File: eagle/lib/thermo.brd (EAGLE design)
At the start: 160 x 100 mm, 16 parts, among them U2 MLX90640ESF-BAB-000-TU

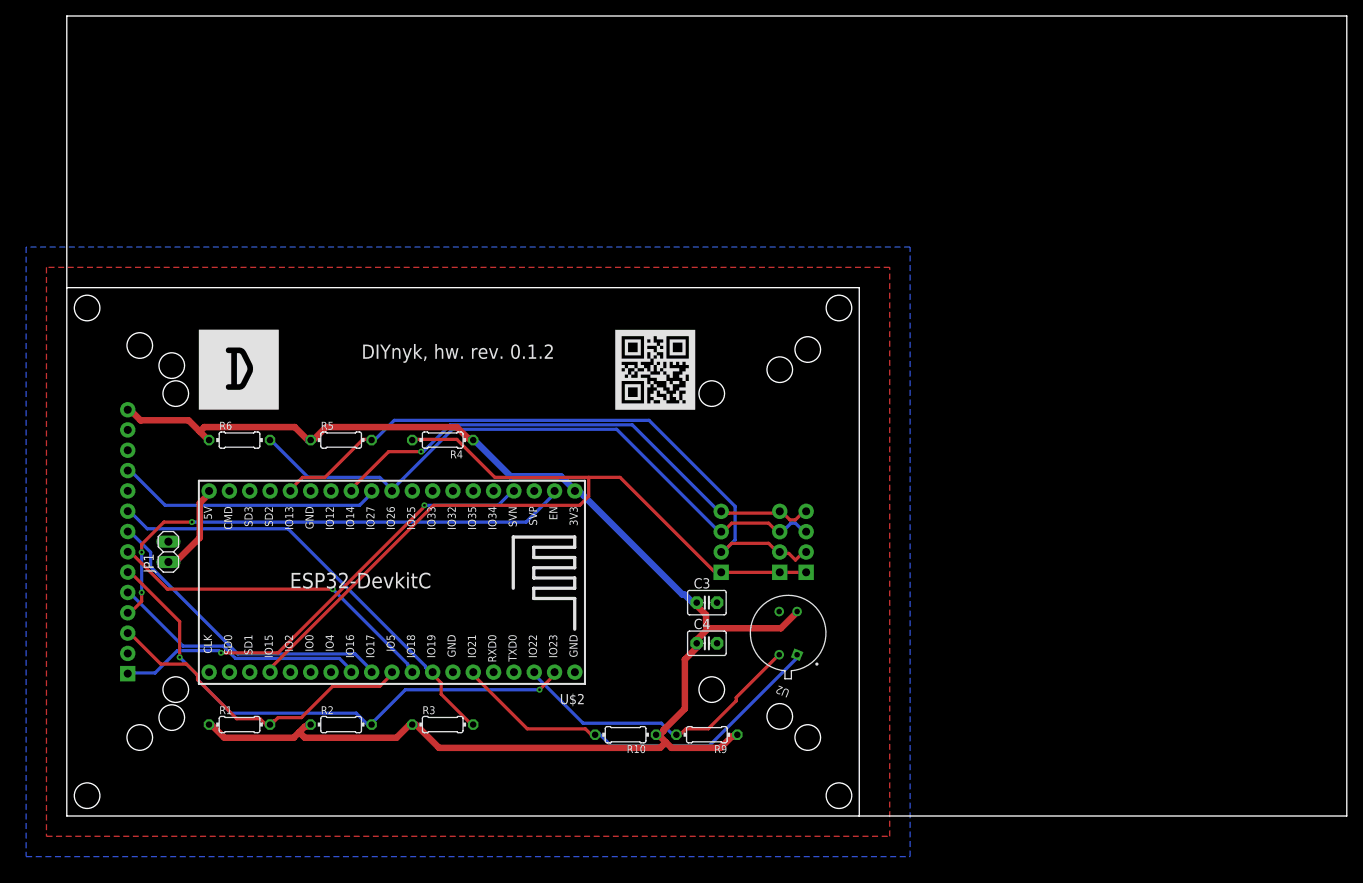
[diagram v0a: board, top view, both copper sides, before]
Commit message: Fixed scheme 0.1.2
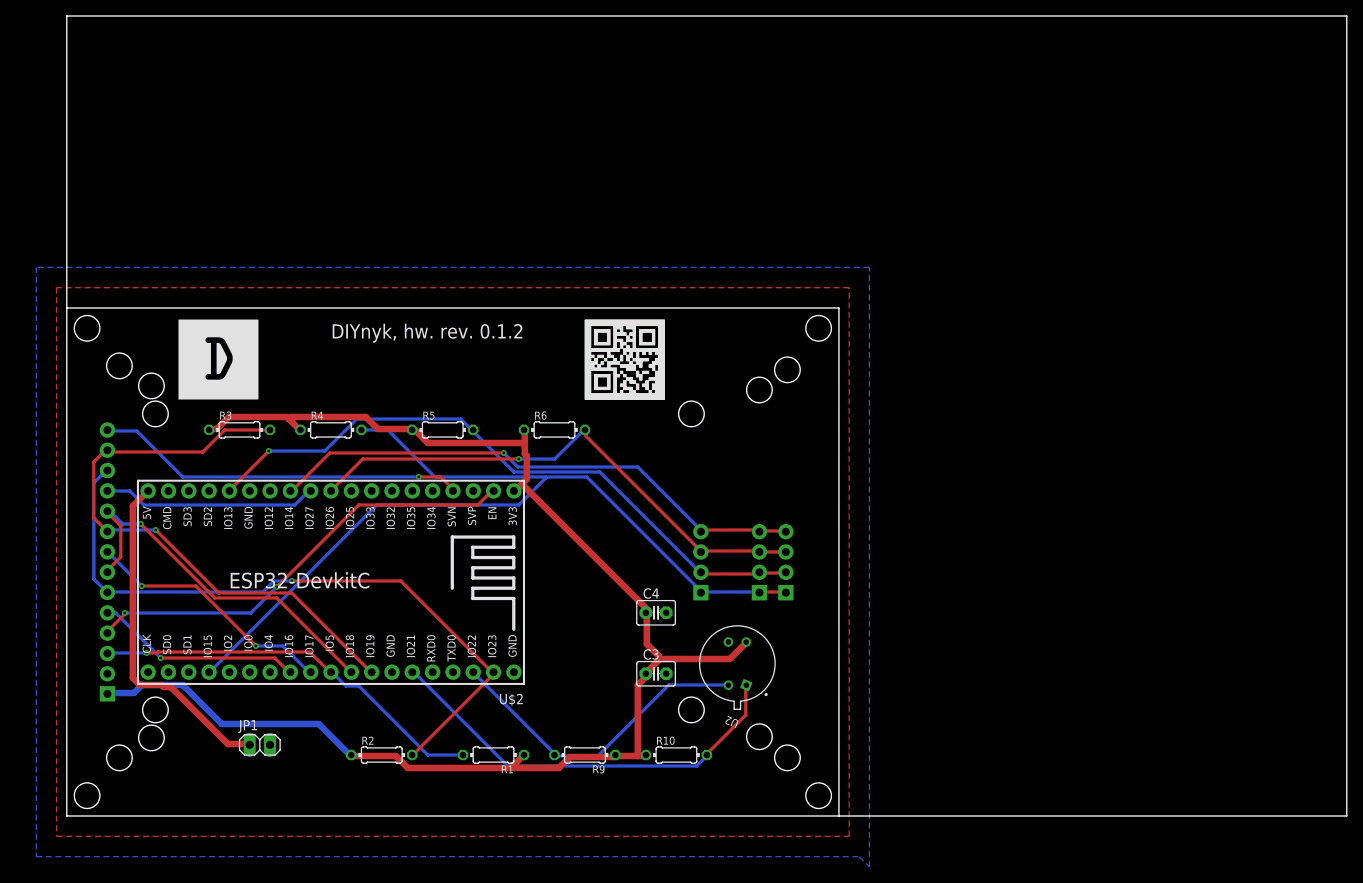
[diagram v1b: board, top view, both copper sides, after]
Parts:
- added U$5: (no value), thermo:QR_10MM
- moved R3 44.7 mm to (21.6, 48.3)
- moved R6 39.4 mm to (61.0, 48.3)
- moved R1 32.0 mm to (53.3, 7.62), turned to 180 degrees
- moved JP1 26.7 mm to (24.1, 8.89), turned to 0 degrees
- moved R9 15.5 mm to (64.8, 7.62)
- moved R4 14.0 mm to (33.0, 48.3), turned to 0 degrees
- moved R5 12.8 mm to (47.0, 48.3)
- moved C3 10.9 mm to (73.7, 17.8)
- moved U$2 7.62 mm to (33.0, 29.2)
- moved C4 7.41 mm to (73.7, 25.4)
- moved U2 7.41 mm to (83.8, 19.1)
- moved R10 6.84 mm to (76.2, 7.62), turned to 0 degrees
- moved R2 6.35 mm to (39.4, 7.62)
- moved U$4 4.02 mm to (64.8, 52.1)
- moved U$1 3.59 mm to (5.08, 48.3)
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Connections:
- net 3V3: now also U$1.VCC!; no longer U$1.TOUCH_IRQ
- net TOUCH_IRQ: now also U$1.TOUCH_IRQ; no longer U$1.VCC!
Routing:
- net +5V: track 11.5 -> 42.3 mm
- net TFT_MISO: track 55.3 -> 73.8 mm, vias 0 -> 1
- net TFT_MOSI: track 67.1 -> 85.0 mm, vias 2 -> 1
- net SD_MISO: track 80.2 -> 67.2 mm, vias 0 -> 1
- net TOUCH_IRQ: track 58.1 -> 46.6 mm, vias 2 -> 1
- net TFT_CS: track 41.0 -> 50.0 mm, vias 0 -> 1
- net 3V3: track 190.6 -> 181.8 mm
- net TFT_RESET: track 64.0 -> 56.0 mm, vias 3 -> 2
- net TFT_LED: track 39.0 -> 31.7 mm, vias 0 -> 2
- net SD_CS: track 107.7 -> 114.1 mm
- net TFT_DC: track 32.2 -> 26.0 mm, vias 0 -> 1
- net TOUCH_CS: track 33.1 -> 27.0 mm
- net TFT_SCK: track 42.0 -> 47.9 mm
- net SDA: track 49.6 -> 53.1 mm
- net SD_SCK: track 66.0 -> 68.6 mm
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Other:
- outline, holes or cut-outs redrawn

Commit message: comleted
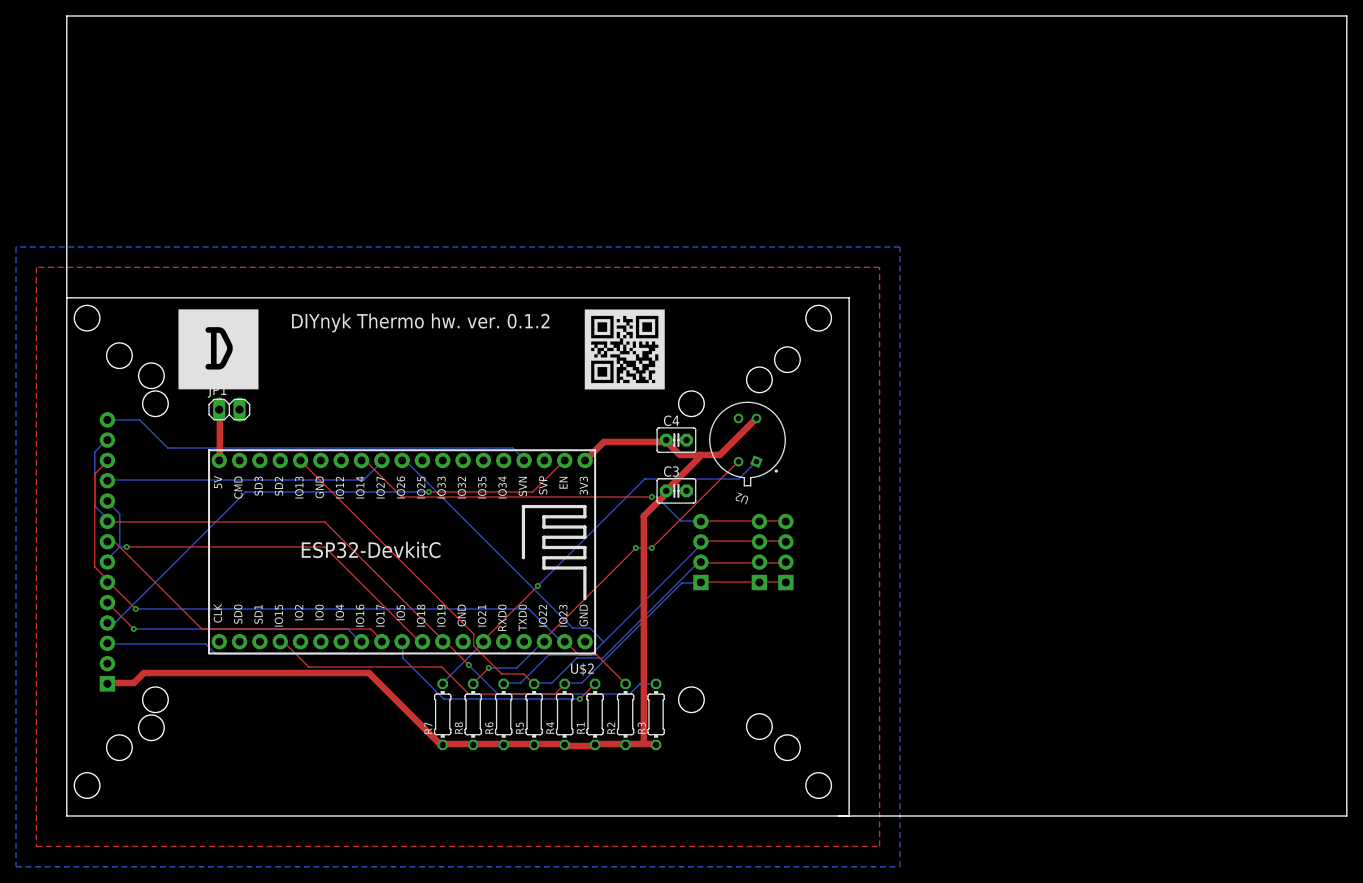
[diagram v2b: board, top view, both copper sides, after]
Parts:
- removed R10, R9: 1K, rcl:0204/7
- removed U$5: (no value), thermo:QR_10MM
- added R7, R8: 1K, rcl:0204/7
- U$1: value ILI9341_DISPLAY_SD_MODULE -> (none); device thermo:ILI9341_DISPLAY_SD_MODULE -> thermo:DIYNYK_10MM
- U$3: value (none) -> ILI9341_DISPLAY_SD_MODULE; device thermo:DIYNYK_10MM -> thermo:ILI9341_DISPLAY_SD_MODULE
- moved R3 63.1 mm to (73.7, 12.7), turned to 90 degrees
- moved R4 46.0 mm to (62.2, 12.7), turned to 90 degrees
- moved JP1 42.1 mm to (20.3, 50.8)
- moved R5 37.4 mm to (58.4, 12.7), turned to 90 degrees
- moved R6 36.1 mm to (54.6, 12.7), turned to 90 degrees
- moved R2 30.9 mm to (69.8, 12.7), turned to 90 degrees
- moved U2 28.0 mm to (85.1, 47.0)
- moved C3 23.0 mm to (76.2, 40.6)
- moved C4 21.7 mm to (76.2, 47.0)
- moved R1 13.7 mm to (66.0, 12.7), turned to 90 degrees
- moved U$1 10.2 mm to (14.0, 53.3), flipped to the top, turned to 0 degrees
- moved U$2 9.67 mm to (41.9, 33.0)
- moved U$3 9.25 mm to (5.08, 49.5), flipped to the bottom, turned to 90 degrees
- moved U$4 1.27 mm to (64.8, 53.3)
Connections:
- net 3V3: now also R7.1, R8.1, U$3.VCC; no longer R10.1, R9.1, U$1.VCC!
- net GND: now also U$3.GND; no longer U$1.GND
- net SCL: now also R8.2; no longer R9.2
- net SDA: now also R7.2; no longer R10.2
- net SD_CS: now also U$3.SD_CS_24, U$3.SD_CS_28, U$3.SD_CS_32; no longer U$1.SD_CS_24, U$1.SD_CS_28, U$1.SD_CS_32
- net SD_MISO: now also U$3.SD_MISO_24, U$3.SD_MISO_28, U$3.SD_MISO_32; no longer U$1.SD_MISO_24, U$1.SD_MISO_28, U$1.SD_MISO_32
- net SD_MOSI: now also U$3.SD_MOSI_24, U$3.SD_MOSI_28, U$3.SD_MOSI_32; no longer U$1.SD_MOSI_24, U$1.SD_MOSI_28, U$1.SD_MOSI_32
- net SD_SCK: now also U$3.SD_SCK_24, U$3.SD_SCK_28, U$3.SD_SCK_32; no longer U$1.SD_SCK_24, U$1.SD_SCK_28, U$1.SD_SCK_32
- net TFT_CS: now also U$3.TFT_CS; no longer U$1.TFT_CS
- net TFT_DC: now also U$3.TFT_DC; no longer U$1.TFT_DC
- net TFT_LED: now also U$3.TFT_LED; no longer U$1.TFT_LED
- net TFT_MISO: now also U$3.TFT_SDO(MISO), U$3.TOUCH_DO; no longer U$1.TFT_SDO(MISO), U$1.TOUCH_DO
- net TFT_MOSI: now also U$3.TFT_SDI(MOSI), U$3.TOUCH_DIN; no longer U$1.TFT_SDI(MOSI), U$1.TOUCH_DIN
- net TFT_RESET: now also U$3.TFT_RESET; no longer U$1.TFT_RESET
- net TFT_SCK: now also U$3.TFT_SCK, U$3.TOUCH_CLK(SCK); no longer U$1.TFT_SCK, U$1.TOUCH_CLK(SCK)
- net TOUCH_CS: now also U$3.TOUCH_CS; no longer U$1.TOUCH_CS
- net TOUCH_IRQ: now also U$3.TOUCH_IRQ; no longer U$1.TOUCH_IRQ
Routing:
- net 3V3: track 181.8 -> 137.6 mm
- net SD_CS: track 114.1 -> 71.9 mm
- net +5V: track 42.3 -> 6.43 mm
- net TFT_CS: track 50.0 -> 66.5 mm
- net TFT_MISO: track 73.8 -> 90.1 mm
- net SD_SCK: track 68.6 -> 56.4 mm
- net SD_MISO: track 67.2 -> 77.8 mm, vias 1 -> 0
- net TFT_RESET: track 56.0 -> 65.6 mm, vias 2 -> 1
- net TOUCH_CS: track 27.0 -> 35.6 mm
- net TFT_LED: track 31.7 -> 39.7 mm, vias 2 -> 0
- net TFT_DC: track 26.0 -> 33.8 mm
- net TOUCH_IRQ: track 46.6 -> 54.4 mm, vias 1 -> 0
- net SCL: track 40.1 -> 44.9 mm, vias 0 -> 3
- net TFT_SCK: track 47.9 -> 51.7 mm
- net TFT_MOSI: track 85.0 -> 87.2 mm
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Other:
- outline, holes or cut-outs redrawn
- board text added: "DIYnyk Thermo hw. ver. 0.1.2"
- board text removed: "DIYnyk, hw. rev. 0.1.2"
